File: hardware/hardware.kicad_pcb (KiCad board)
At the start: 2 copper layers, 55 parts, among them J101 VIN, J102 BAT, J103 DISPLAY, J104 EXT, J105 VIN, J106 SENSOR_DHT, J107 solo, SW101 BOOT, U101 LM324, U102 TP4056, U103 DW01, U104 FS8205A, U105 AMS1117-3.3, U106 ESP32-WROOM-32

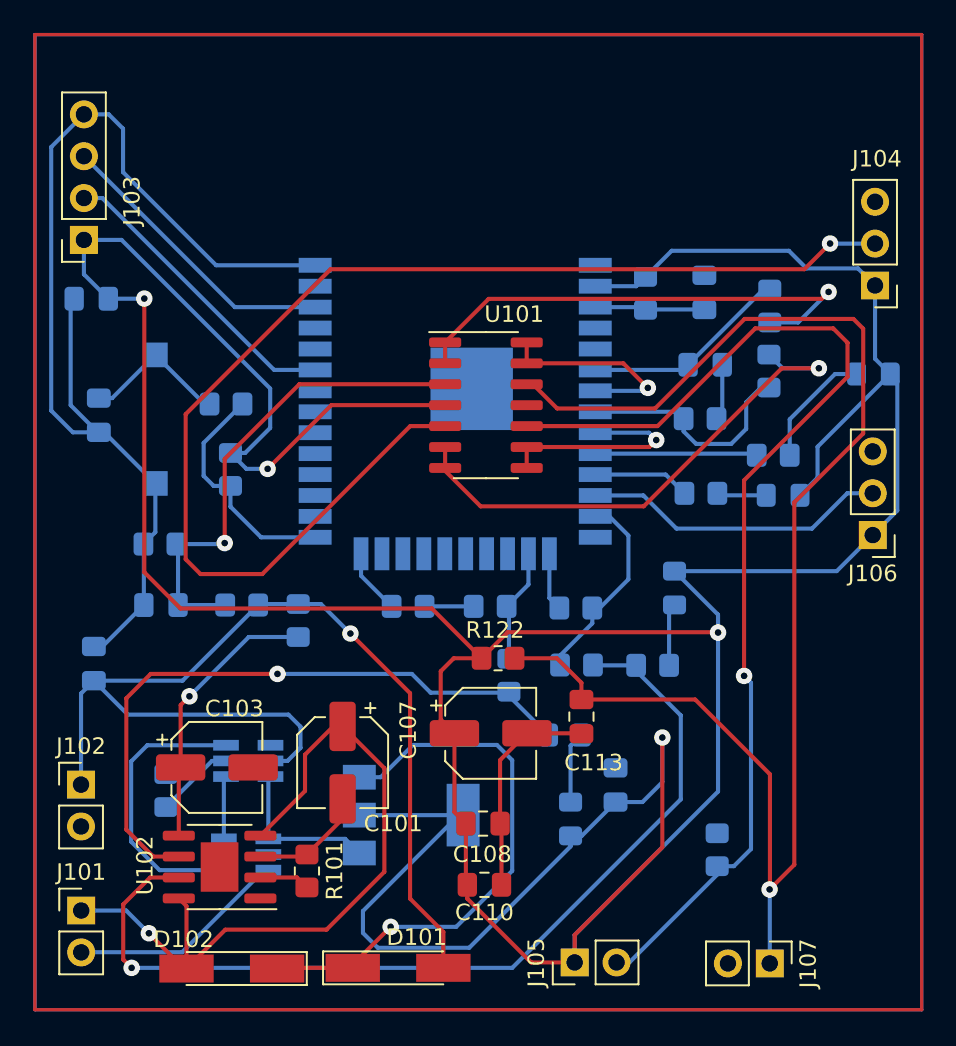
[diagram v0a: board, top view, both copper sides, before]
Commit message: pcb
finalizado
- precisa revisar pcb e esquemático
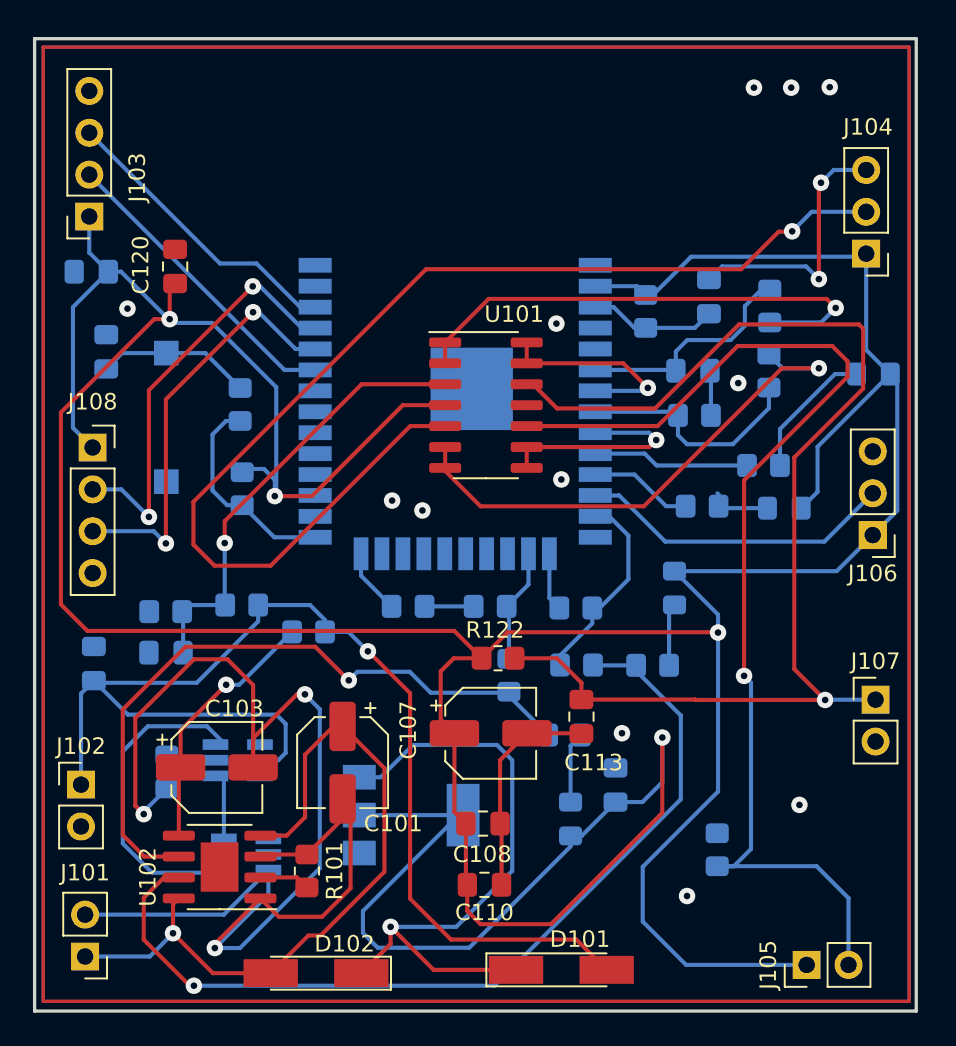
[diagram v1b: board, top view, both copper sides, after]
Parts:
- added C120: 100nF, Capacitor_SMD:C_0805_2012Metric_Pad1.18x1.45mm_HandSolder, F.Cu at (103.5, 111.1)
- added J108: TX_RX, Connector_PinSocket_2.54mm:PinSocket_1x04_P2.54mm_Vertical, F.Cu at (98.5, 122.0)
- moved J107 17.2 mm to (146.0, 137.4), turned to 0 degrees
- moved J105 14.1 mm to (141.9, 153.4)
- moved D101 9.91 mm to (127.0, 153.8)
- moved D102 5.12 mm to (112.1, 154.0)
- moved R106 4.12 mm to (103.0, 132.0)
- moved C109 3.88 mm to (99.3, 116.2), turned to -90 degrees
- moved C106 2.91 mm to (103.0, 134.5)
- moved J101 2.80 mm to (98.1, 152.9), turned to 180 degrees
- moved J104 2.00 mm to (145.5, 110.3)
- moved C111 1.64 mm to (98.4, 111.4)
- moved J103 1.46 mm to (98.3, 108.0)
- moved R107 1.37 mm to (107.6, 124.5)
- moved R102 1.13 mm to (103.0, 141.7), turned to 90 degrees
- moved R104 1.10 mm to (132.1, 113.8)
- moved R103 0.93 mm to (111.6, 133.2), turned to 180 degrees
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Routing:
- net GND1: track 20.6 -> 89.9 mm, vias 0 -> 3
- net GND: track 100.4 -> 39.3 mm, vias 0 -> 14
- net /RX: track 0.00 -> 25.7 mm, vias 0 -> 2
- net +3V3: track 265.4 -> 291.0 mm
- net /TX: track 0.00 -> 25.5 mm, vias 0 -> 2
- net Net-(C113-Pad2): track 90.4 -> 71.8 mm
- net BAT+: track 64.6 -> 73.5 mm
- net Net-(J104-Pad2): track 74.8 -> 70.0 mm
- net Net-(D101-Pad1): track 34.0 -> 38.2 mm
- net /VBAT: track 29.9 -> 27.3 mm
- net Net-(U103-Pad3): track 17.4 -> 19.9 mm
- net Net-(J105-Pad2): track 67.1 -> 69.5 mm
- net /CHRG: track 57.6 -> 55.5 mm
- net /STDBY: track 39.8 -> 41.8 mm
- net Net-(R102-Pad2): track 4.81 -> 3.07 mm
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- added copper zone on B.Cu, net GND
- added copper zone on F.Cu, net GND
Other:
- board outline added: 53.5 x 59 mm
